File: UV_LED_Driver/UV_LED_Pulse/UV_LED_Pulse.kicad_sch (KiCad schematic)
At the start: 21 parts, among them J1 PWR/Signal, Q1 BC817, Q2 2N7002

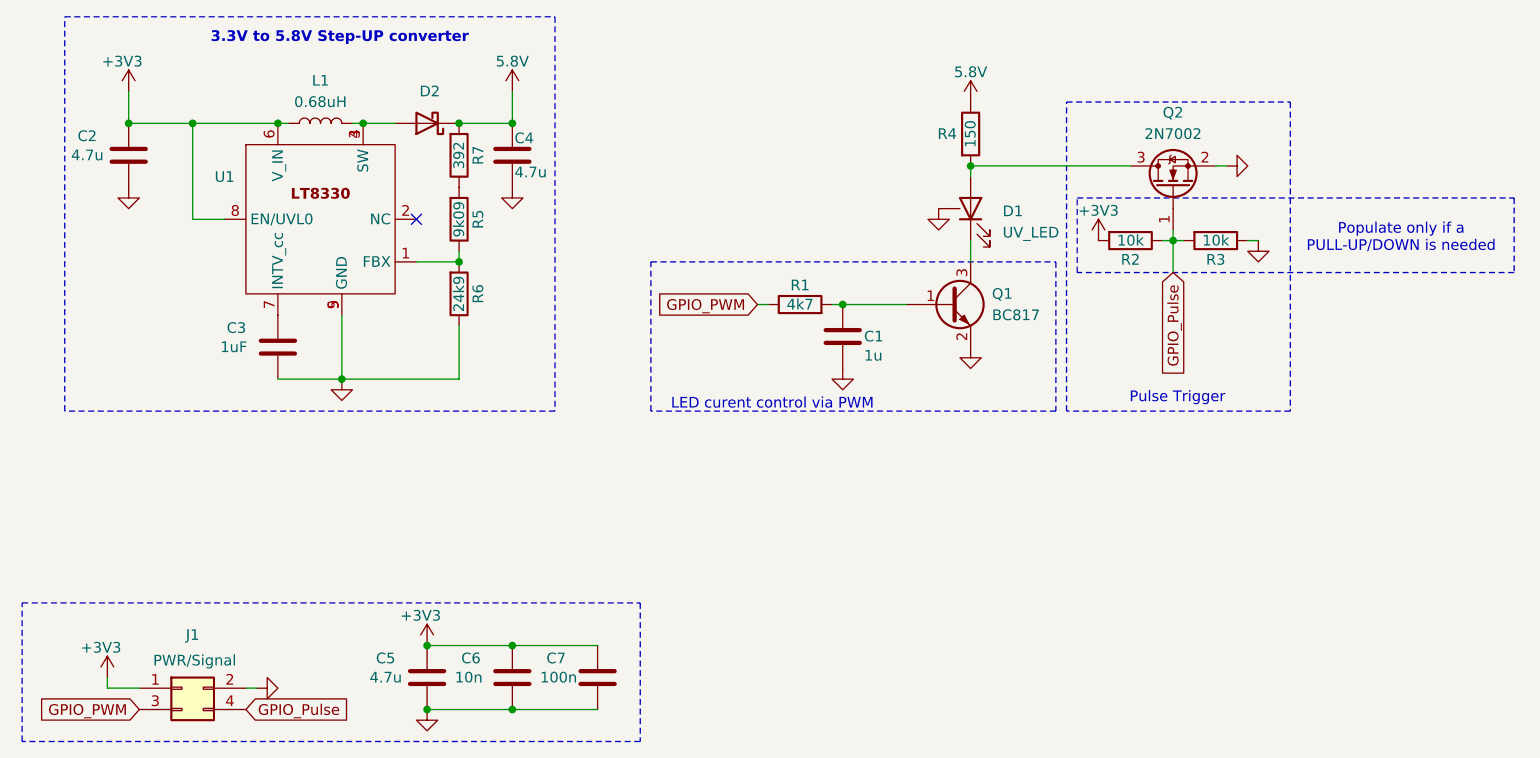
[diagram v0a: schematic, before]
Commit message: .
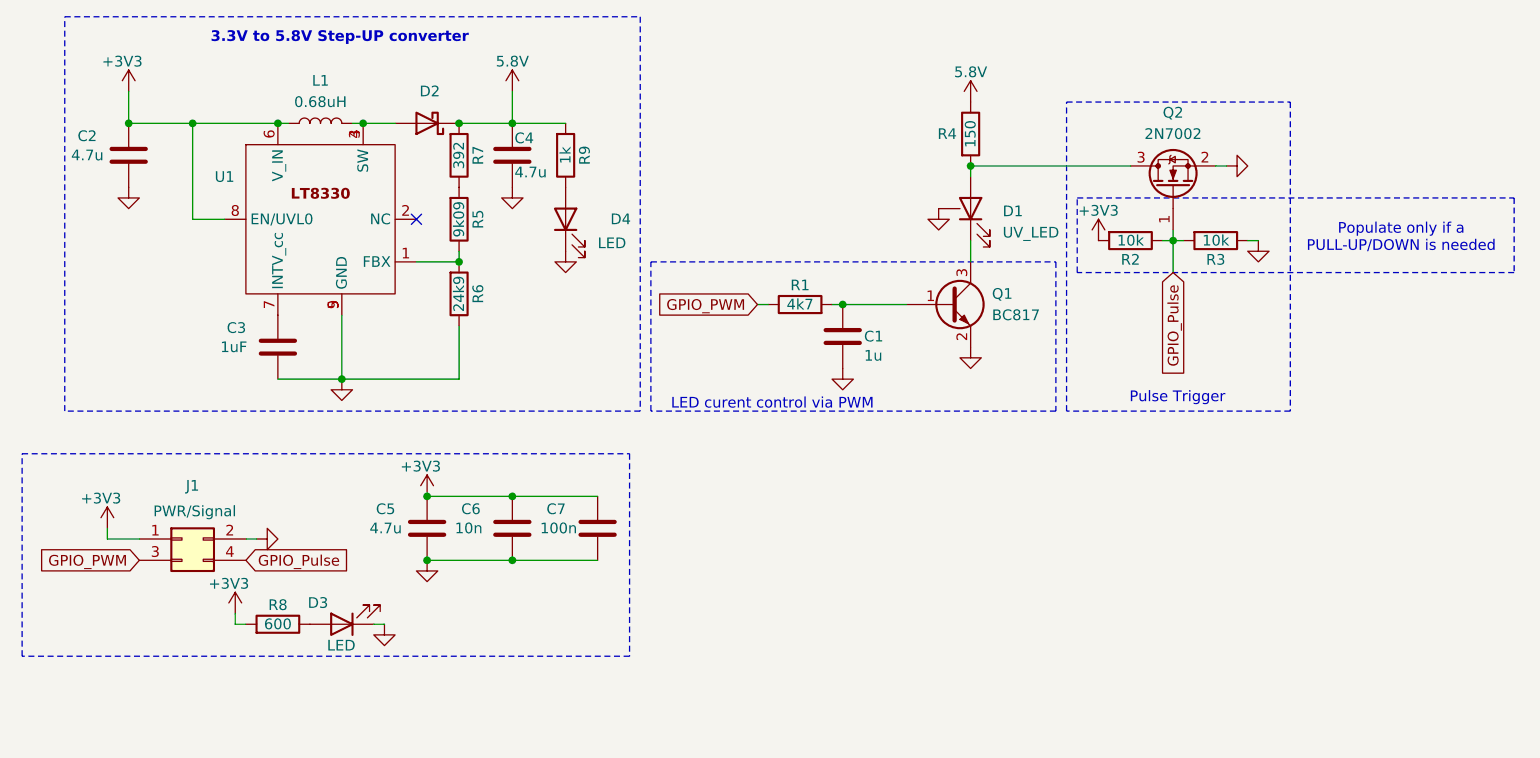
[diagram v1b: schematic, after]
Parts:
- added D3, D4: LED, LED_SMD:LED_0603_1608Metric, symbol Device:LED
- added R8: 600, Resistor_SMD:R_0603_1608Metric, symbol Device:R
- added R9: 1k, Resistor_SMD:R_0603_1608Metric, symbol Device:R
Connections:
- net +3V3: now also R8.2
- net 5.8V: now also R9.2
- net GND: now also D3.1 (K), D4.1 (K)
- new net: D3.2 (A), R8.1
- new net: D4.2 (A), R9.1
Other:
- moved on the sheet: C5, C6, C7, J1
